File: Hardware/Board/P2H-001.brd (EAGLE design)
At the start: 45 x 45 mm, 15 parts, among them IC1 74LS07N, IC2 LTC485N

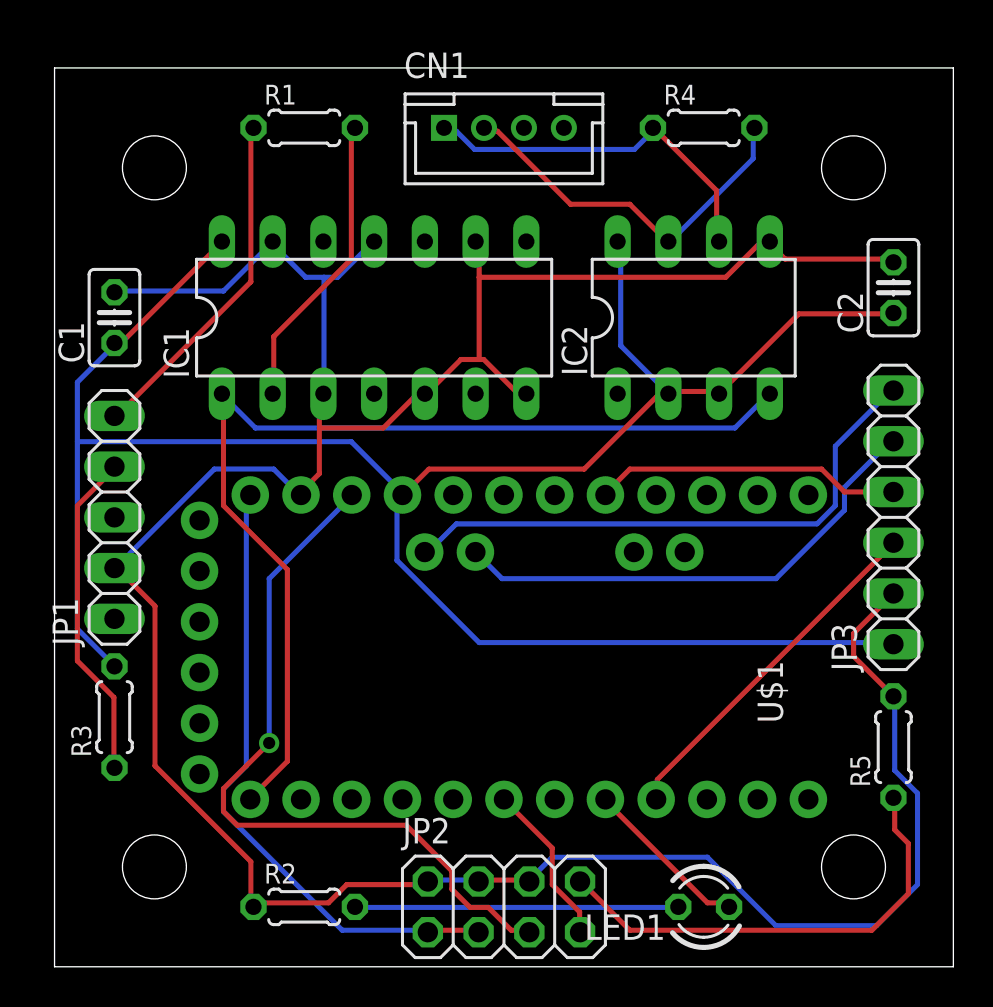
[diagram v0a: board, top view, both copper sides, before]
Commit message: Clean up.
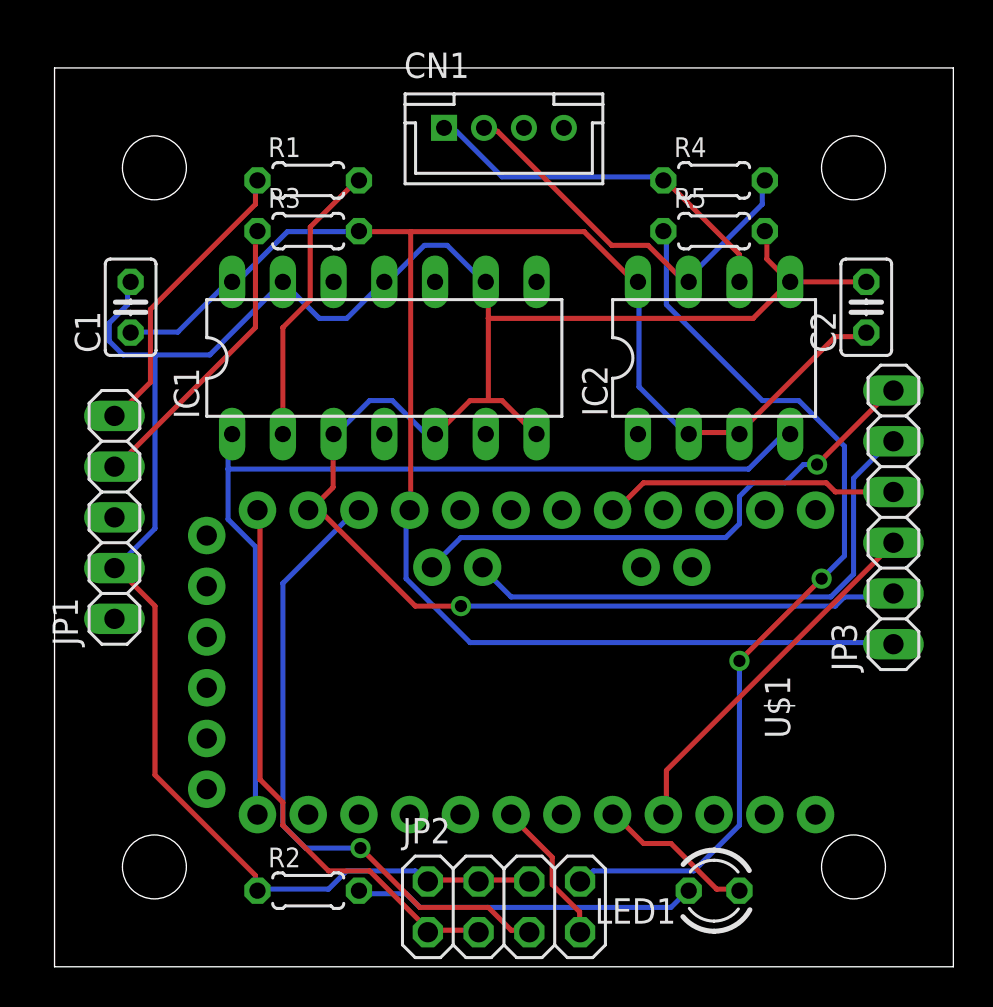
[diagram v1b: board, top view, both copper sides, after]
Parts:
- moved R5 27.3 mm to (33.0, 36.8), turned to 0 degrees
- moved R3 26.2 mm to (12.7, 36.8), turned to 0 degrees
- moved R4 2.68 mm to (33.0, 39.4)
- moved R1 2.64 mm to (12.7, 39.4)
- moved IC2 2.26 mm to (33.0, 30.5)
- moved IC1 2.08 mm to (16.5, 30.5)
- moved C2 1.68 mm to (40.6, 33.0)
- moved C1 0.96 mm to (3.81, 33.0)
- moved LED1 0.96 mm to (33.0, 3.81)
- moved U$1 0.84 mm to (22.9, 15.2)
- moved R2 0.83 mm to (12.7, 3.81)
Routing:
- net N$5: track 23.3 -> 45.9 mm, vias 0 -> 2
- net VCC: track 109.8 -> 91.7 mm
- net N$6: track 36.8 -> 32.0 mm
- net N$9: track 31.8 -> 28.5 mm
- net GND: track 152.7 -> 150.1 mm, vias 0 -> 1
- net N$1: track 51.3 -> 48.7 mm
- net N$7: track 17.3 -> 14.8 mm
- net N$11: track 25.0 -> 27.2 mm
- net N$3: track 16.6 -> 14.8 mm
- net N$19: track 19.1 -> 20.4 mm
- net N$13: track 16.2 -> 17.2 mm
- net N$14: track 28.5 -> 27.6 mm, vias 0 -> 1
- net N$8: track 8.22 -> 7.31 mm
- net N$2: track 15.0 -> 14.3 mm
- net N$4: track 15.5 -> 14.8 mm
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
